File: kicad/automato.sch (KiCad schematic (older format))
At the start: 82 parts, among them J1 USB_C_Receptacle, J10 QWIIC 0, J12 STEMMA 0, J2 LiPo, J3 Conn_01x07_Male, J4 Screw_Terminal_01x14, J5 USB_C_Receptacle, J6 Conn_Coaxial, J7 1-WIRE, J8 Micro_SD_Card_Det, J9 UART2, M1 eink-module, Q1 Q_NPN_BCE, Q2 Q_NPN_BCE, Q3 DMG3415U, Q4 Q_DUAL_NMOS_S1G1D2S2G2D1, Q6 Q_DUAL_NMOS_S1G1D2S2G2D1, Q7 Q_DUAL_NMOS_S1G1D2S2G2D1, SW1 SW_Push, SW2 SW_Push, SW3 SW_SPDT, U1 CP2104, U2 AP2112K-3.3, U3 RFM95W-915S2, U4 ESP32-WROOM-32D, U5 SHTC3, U6 MCP73831-2-OT, U7 MP2452, U8 ESP32-WROOM-DA

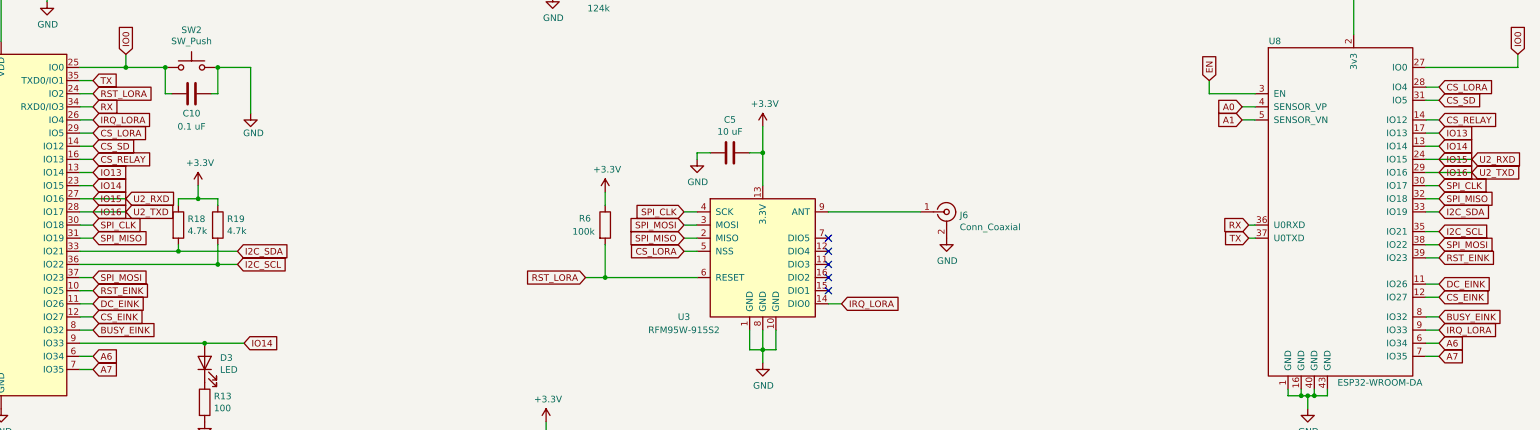
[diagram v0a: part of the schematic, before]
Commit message: playing with pins
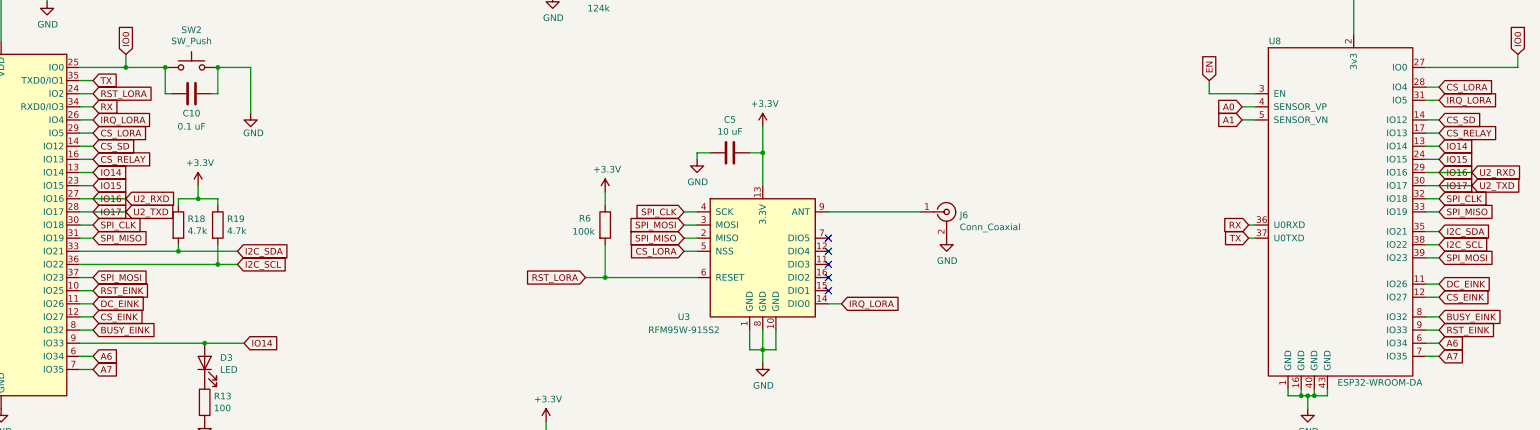
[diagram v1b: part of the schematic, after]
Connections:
- net CS_RELAY: now also U8.17 (IO13); no longer U8.14 (IO12)
- net CS_SD: now also U8.14 (IO12); no longer U8.31 (IO5)
- net I2C_SCL: now also U8.38 (IO22); no longer U8.35 (IO21)
- net I2C_SDA: now also U8.35 (IO21); no longer U8.33 (IO19)
- net IO13: no longer U4.13 (IO14), U8.17 (IO13)
- net IO14: now also U4.13 (IO14); no longer U4.23 (IO15)
- net IO15: now also U4.23 (IO15); no longer JP1.3 (B), Q6.1 (S), U4.27 (IO16)
- net IO16: now also JP1.3 (B), Q6.1 (S), U4.27 (IO16); no longer JP2.3 (B), Q6.4 (S), U4.28 (IO17)
- net IRQ_LORA: now also U8.31 (IO5); no longer U8.9 (IO33)
- net RST_EINK: now also U8.9 (IO33); no longer U8.39 (IO23)
- net SPI_CLK: now also U8.32 (IO18); no longer U8.30 (IO17)
- net SPI_MISO: now also U8.33 (IO19); no longer U8.32 (IO18)
- net SPI_MOSI: now also U8.39 (IO23); no longer U8.38 (IO22)
- new net IO17: JP2.3 (B), Q6.4 (S), U4.28 (IO17), U8.30 (IO17)
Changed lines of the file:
@@
 CS_SD
 Text GLabel 9650 5850 2    50   Input ~ 0
+IO17
+Text GLabel 9650 5550 2    50   Input ~ 0
+IO14
+Text GLabel 9650 5650 2    50   Input ~ 0
+IO15
+Text GLabel 9650 5750 2    50   Input ~ 0
 IO16
-Text GLabel 9650 5550 2    50   Input ~ 0
-IO13
-Text GLabel 9650 5650 2    50   Input ~ 0
-IO14
-Text GLabel 9650 5750 2    50   Input ~ 0
-IO15
 Text GLabel 9900 5850 2    50   Input ~ 0
 U2_TXD
@@
 Text GLabel 19900 6500 2    50   Input ~ 0
 CS_EINK
+Text GLabel 19900 6750 2    50   Input ~ 0
+RST_EINK
+Wire Wire Line
+	19800 6750 19900 6750
+Wire Wire Line
+	19800 6200 19900 6200
 Text GLabel 19900 6200 2    50   Input ~ 0
-RST_EINK
-Wire Wire Line
-	19800 6200 19900 6200
-Wire Wire Line
-	19800 6100 19900 6100
+SPI_MOSI
 Text GLabel 19900 6100 2    50   Input ~ 0
-SPI_MOSI
+I2C_SCL
 Text GLabel 19900 6000 2    50   Input ~ 0
-I2C_SCL
-Text GLabel 19900 5850 2    50   Input ~ 0
 I2C_SDA
 Wire Wire Line
@@
 IO16
 Wire Wire Line
+	19800 5850 19900 5850
+Wire Wire Line
 	19800 5750 19900 5750
-Wire Wire Line
-	19800 5650 19900 5650
+Text GLabel 19900 5850 2    50   Input ~ 0
+SPI_MISO
 Text GLabel 19900 5750 2    50   Input ~ 0
-SPI_MISO
-Text GLabel 19900 5650 2    50   Input ~ 0
 SPI_CLK
-Wire Wire Line
-	19800 5450 20150 5450
 Text GLabel 19900 5350 2    50   Input ~ 0
 IO14
@@
 Wire Wire Line
 	19800 5350 19900 5350
-Text GLabel 19900 5000 2    50   Input ~ 0
+Text GLabel 19900 5150 2    50   Input ~ 0
 CS_SD
+Text GLabel 19900 5650 2    50   Input ~ 0
+IO17
 Text GLabel 19900 5250 2    50   Input ~ 0
-IO13
-Text GLabel 19900 5150 2    50   Input ~ 0
 CS_RELAY
 Wire Wire Line
@@
 	19800 5150 19900 5150
 Wire Wire Line
+	19800 4900 19900 4900
+Wire Wire Line
 	19800 5000 19900 5000
-Wire Wire Line
-	19800 4900 19900 4900
-Wire Wire Line
-	19800 6750 19900 6750
 Text GLabel 19900 4900 2    50   Input ~ 0
 CS_LORA
-Text GLabel 19900 6750 2    50   Input ~ 0
+Text GLabel 19900 5000 2    50   Input ~ 0
 IRQ_LORA
 Wire Wire Line
@@
 	18900 7250 18950 7250
 $Comp
-L power:+3.3V #PWR?
+L power:+3.3V #PWR0122
 U 1 1 6371B3EA
 P 19250 3700
-F 0 "#PWR?" H 19250 3550 50  0001 C CNN
+F 0 "#PWR0122" H 19250 3550 50  0001 C CNN
 F 1 "+3.3V" H 19265 3873 50  0000 C CNN
 F 2 "" H 19250 3700 50  0001 C CNN
@@
 	1    0    0    -1
 $EndComp
+Text GLabel 20150 5650 2    50   Input ~ 0
+U2_TXD
 Text GLabel 20150 5550 2    50   Input ~ 0
-U2_TXD
-Text GLabel 20150 5450 2    50   Input ~ 0
 U2_RXD
 Text GLabel 10800 6850 2    50   Input ~ 0
 IO14
 Wire Wire Line
+	19800 6100 19900 6100
+Wire Wire Line
 	19800 6000 19900 6000
-Wire Wire Line
-	19800 5850 19900 5850
 $Comp
 L automato-sensor:ESP32-WROOM-DA U8
@@
 Wire Wire Line
 	19250 3700 19250 4500
+Wire Wire Line
+	19800 5450 19900 5450
+Wire Wire Line
+	19800 5650 20150 5650
 $EndSCHEMATC
